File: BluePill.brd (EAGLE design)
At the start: 98.7 x 72.4 mm, 42 parts, among them X1 MST2V

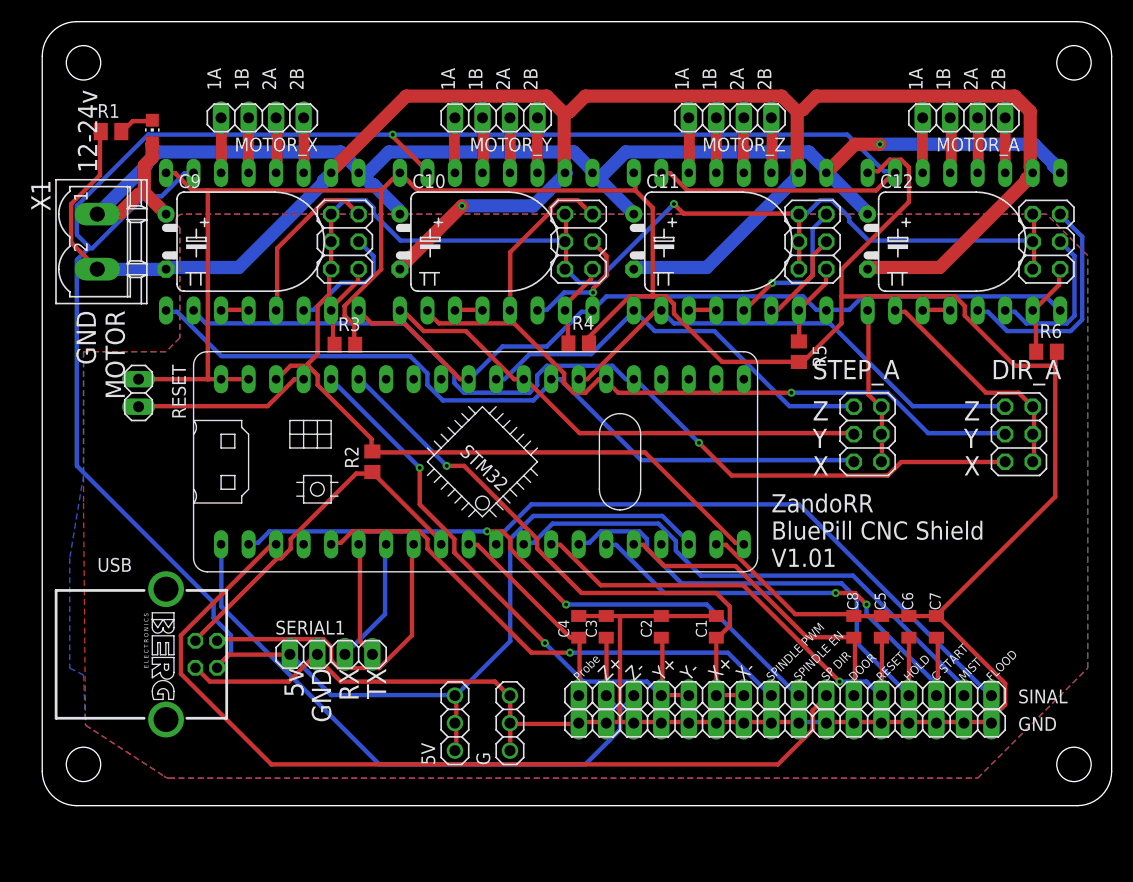
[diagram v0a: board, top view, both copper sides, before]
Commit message: Add files via upload
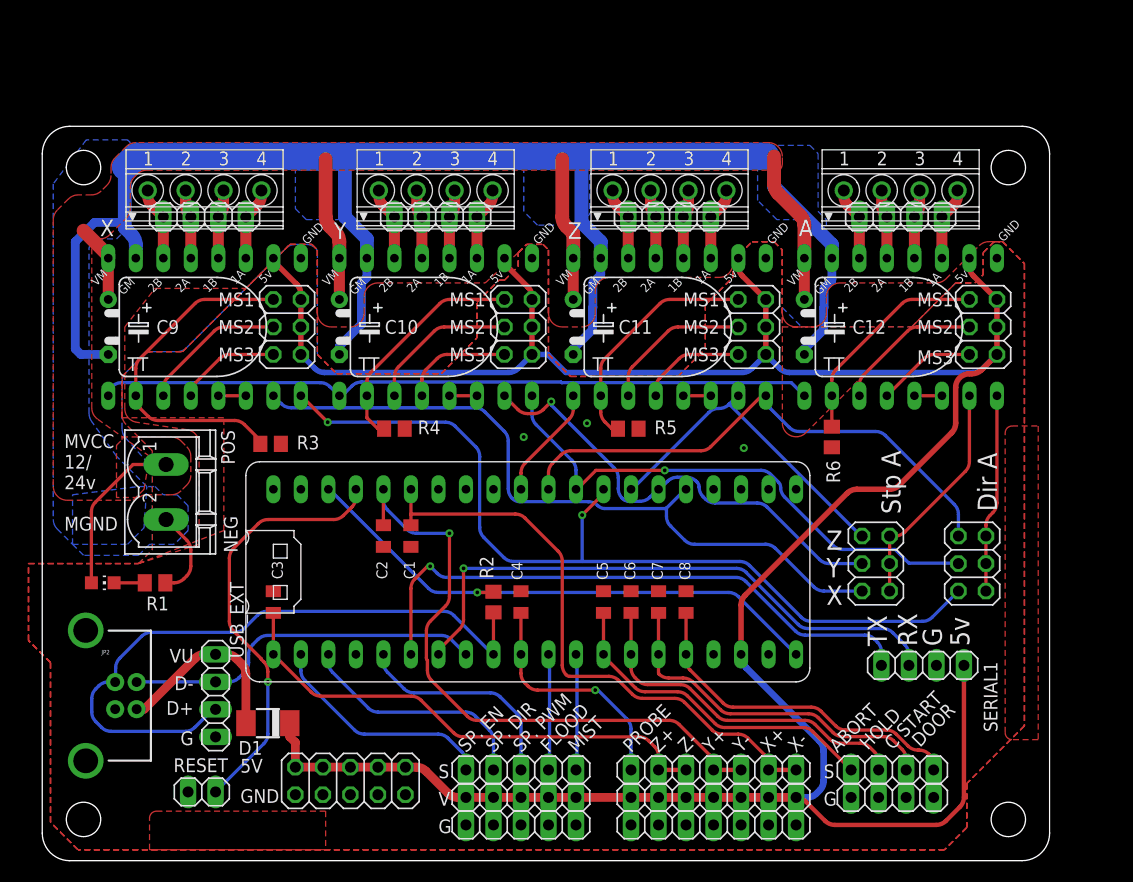
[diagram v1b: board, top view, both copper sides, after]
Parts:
- removed G: (no value), adafruit:1X03
- removed GND, SINAL: (no value), pinhead:1X16
- removed USB: PN61729-S, con-berg:PN61729-S
- added D1: schottky, diode:DO-214AC
- added GND2, SAIDAS: (no value), pinhead:1X05
- added JP1: (no value), pinhead:2X05
- added JP2: (no value), Seeed-Connector:USB4+2-2.5-90D-15.8X12MM
- added JP3, JP4, JP5: (no value), pinhead:1X07
- added JP6, JP7, USB_EXT: (no value), pinhead:1X04
- added X2, X3, X4, X5: 1751264, con-phoenix-350:1751264
- 5V: device adafruit:1X03 -> pinhead:1X05
- moved SERIAL1 54.6 mm to (81.3, 18.0), turned to 180 degrees
- moved LED1 41.9 mm to (5.59, 25.7), turned to 270 degrees
- moved R1 41.9 mm to (10.4, 25.7), turned to 180 degrees
- moved RESET 37.3 mm to (14.7, 6.35), turned to 180 degrees
- moved C3 30.8 mm to (21.3, 23.9)
- moved C1 29.4 mm to (34.0, 30.0), turned to 270 degrees
- moved C2 27.0 mm to (31.5, 30.0), turned to 270 degrees
- moved C6 25.8 mm to (54.4, 23.9)
- moved C5 25.8 mm to (51.8, 23.9)
- moved C7 25.8 mm to (56.9, 23.9)
- moved X1 24.0 mm to (11.4, 34.0)
- moved R6 21.3 mm to (72.9, 39.1), turned to 270 degrees
- moved R4 18.8 mm to (32.5, 39.9)
- moved MSA1 17.8 mm to (77.0, 27.4)
- moved R5 17.3 mm to (54.1, 39.9), turned to 0 degrees
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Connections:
- new net USB5V: D1.A, JP2.VBUS, USB_EXT.1
- net 1A_X: now also X2.4
- net 1B_X: now also X2.3
- net 2A_X: now also X2.2
- net 2B_X: now also X2.1
- net 3V3: no longer MSA.2, MSA.4, MSA.6, MSX.2, MSX.4, MSX.6, MSY.2, MSY.4, MSY.6, MSZ.2, MSZ.4, MSZ.6
- net 5V: now also 5V.4, 5V.5, D1.C, JP1.1, JP1.3, JP1.5, JP1.7, JP1.9, JP3.1, JP3.2, JP3.3, JP3.4, JP3.5, JP3.6, JP3.7, MSA.2, MSA.4, MSA.6, MSX.2, MSX.4, MSX.6, MSY.2, MSY.4, MSY.6, MSZ.2, MSZ.4, MSZ.6; no longer USB.1
- net COOL_FLOOD: now also SAIDAS.4; no longer SINAL.1
- net COOL_MIST: now also SAIDAS.5; no longer SINAL.2
- net CTL_CYCLESTART: now also JP6.3; no longer SINAL.3
- net CTL_FEEDHOLD: now also JP6.2; no longer SINAL.4
- net CTL_RESET: now also JP6.1; no longer SINAL.5
- net CTL_SAFETYDOOR: now also JP6.4; no longer SINAL.6
- net GND: now also GND2.1, GND2.2, GND2.3, GND2.4, GND2.5, JP1.10, JP1.2, JP1.4, JP1.6, JP1.8, JP2.GND, JP4.1, JP4.2, JP4.3, JP4.4, JP4.5, JP4.6, JP4.7, JP7.1, JP7.2, JP7.3, JP7.4, USB_EXT.4; no longer G.1, G.2, G.3, GND.1, GND.10, GND.11, GND.12, GND.13, GND.14, GND.15, GND.16, GND.2, GND.3, GND.4, GND.5, GND.6, GND.7, GND.8, GND.9, USB.4
- net N$21: now also X3.1
- net N$22: now also X3.2
- net N$23: now also X3.3
- net N$24: now also X3.4
- net N$25: now also X4.1
- net N$26: now also X4.2
- net N$27: now also X4.3
- net N$28: now also X4.4
- net N$29: now also X5.1
- net N$30: now also X5.2
- net N$31: now also X5.3
- net N$32: now also X5.4
- net SPINDLE_DIR: now also SAIDAS.2; no longer SINAL.7
- net SPINDLE_ENABLE: now also SAIDAS.1; no longer SINAL.8
- net SPINDLE_PWM: now also SAIDAS.3; no longer SINAL.9
- net USB_DM: now also JP2.D-, USB_EXT.2; no longer USB.2
- net USB_DP: now also JP2.D+, USB_EXT.3; no longer USB.3
- net XLIMIT: now also JP5.1, JP5.2; no longer SINAL.10, SINAL.11
- net YLIMIT: now also JP5.3, JP5.4; no longer SINAL.12, SINAL.13
- net ZLIMIT: now also JP5.5, JP5.6; no longer SINAL.14, SINAL.15
- net Z_PROBE: now also JP5.7; no longer SINAL.16
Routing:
- net GND: track 347.2 -> 0.00 mm, vias 0 -> 3
- net 3V3: track 156.0 -> 50.8 mm
- net VMOT: track 126.7 -> 63.6 mm, vias 1 -> 0
- net SPINDLE_DIR: track 82.6 -> 22.0 mm
- net TX1: track 10.7 -> 55.1 mm, vias 0 -> 1
- net COOL_FLOOD: track 54.8 -> 10.8 mm
- net RX1: track 11.8 -> 54.2 mm, vias 0 -> 1
- net COOL_MIST: track 49.1 -> 10.8 mm
- net SPINDLE_ENABLE: track 58.1 -> 21.3 mm, vias 2 -> 0
- net USB_DP: track 32.8 -> 61.1 mm
- net SPINDLE_PWM: track 48.0 -> 20.4 mm, vias 1 -> 0
- net GNDM: track 185.1 -> 157.6 mm, vias 1 -> 0
- net ARDU_RESET: track 16.3 -> 40.1 mm, vias 0 -> 1
- net MS1: track 8.45 -> 31.7 mm
- net USB5V: track 0.00 -> 17.5 mm
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- added copper zone on layer 16, net GNDM
- added copper zone on layer 1, net N$7
- added copper zone on layer 1, net N$8
- added copper zone on layer 1, net VMOT
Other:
- board size 98.7 x 72.4 mm -> 93 x 67.8 mm
- board text added: "12/ 24v"
- board text added: "5V"
- board text added: "A"
- board text added: "ABORT"
- board text added: "BluePill CNC Base"
- board text added: "D+"
- board text added: "D-"
- board text added: "Dir A"
- board text added: "G"
- board text added: "GM"
- board text added: "MGND"
- board text added: "MS1"
- board text added: "MS2"
- board text added: "MS3"
- board text added: "MVCC"
- board text added: "NEG"
- board text added: "Name here"
- board text added: "POS"
- board text added: "PROBE"
- board text added: "S"
- board text added: "SP. DIR"
- board text added: "SP. EN"
- board text added: "SP. PWM"
- board text added: "Stp A"
- board text added: "V"
- board text added: "VM"
- board text added: "VU"
- board text removed: "12-24v"
- board text removed: "DIR_A"
- board text removed: "GND MOTOR"
- board text removed: "Probe"
- board text removed: "RESET"
- board text removed: "SP DIR"
- board text removed: "SPINDLE EN"
- board text removed: "SPINDLE PWM"
- board text removed: "STEP_A"
- board text removed: "ZandoRR BluePill CNC Shield V1.01"
